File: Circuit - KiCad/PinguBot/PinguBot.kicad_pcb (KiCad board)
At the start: 2 copper layers, 96.3 x 104.8 mm, 26 parts, among them J1 Jack-DC, J2 Conn_01x08_Pin, J3 Conn_01x08_Pin, U1 LM386, U3 LM7805_TO220, U4 TSOP45xx, U5 ESP32_DEVKITC

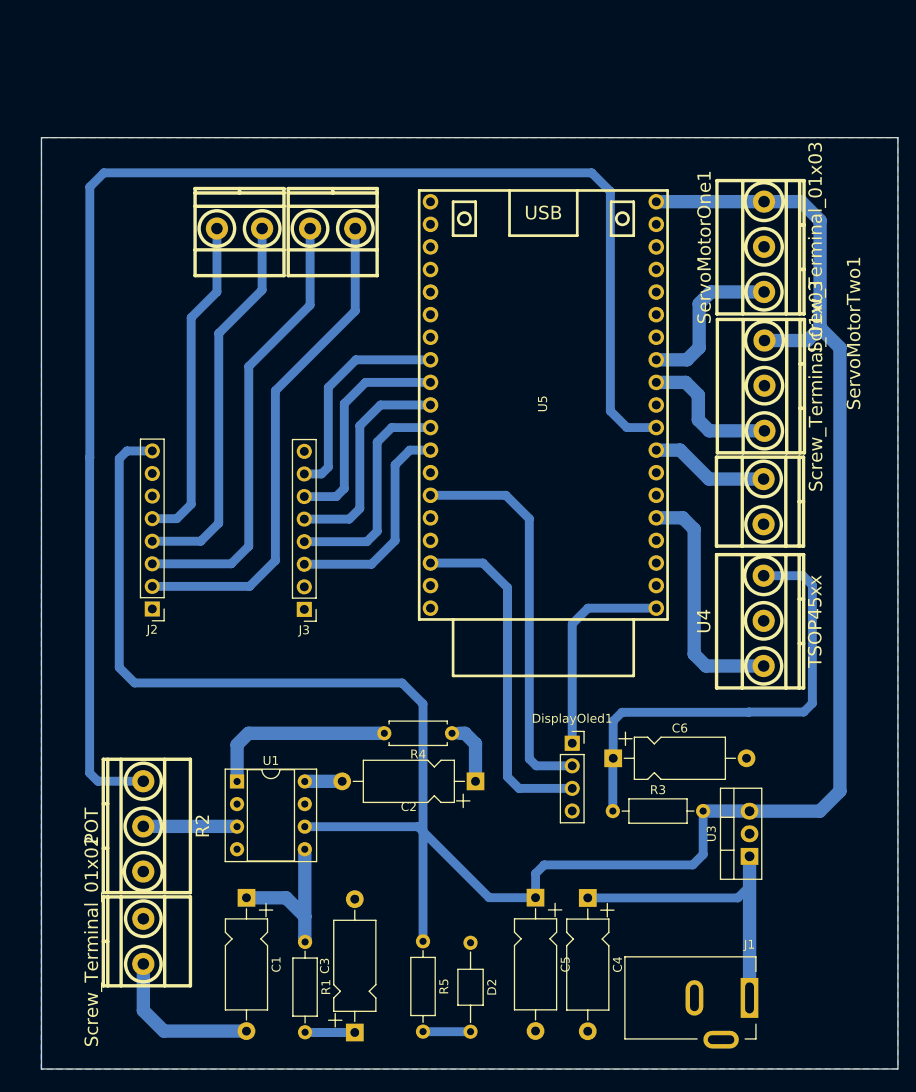
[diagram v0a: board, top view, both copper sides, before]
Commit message: Circuit Improvement
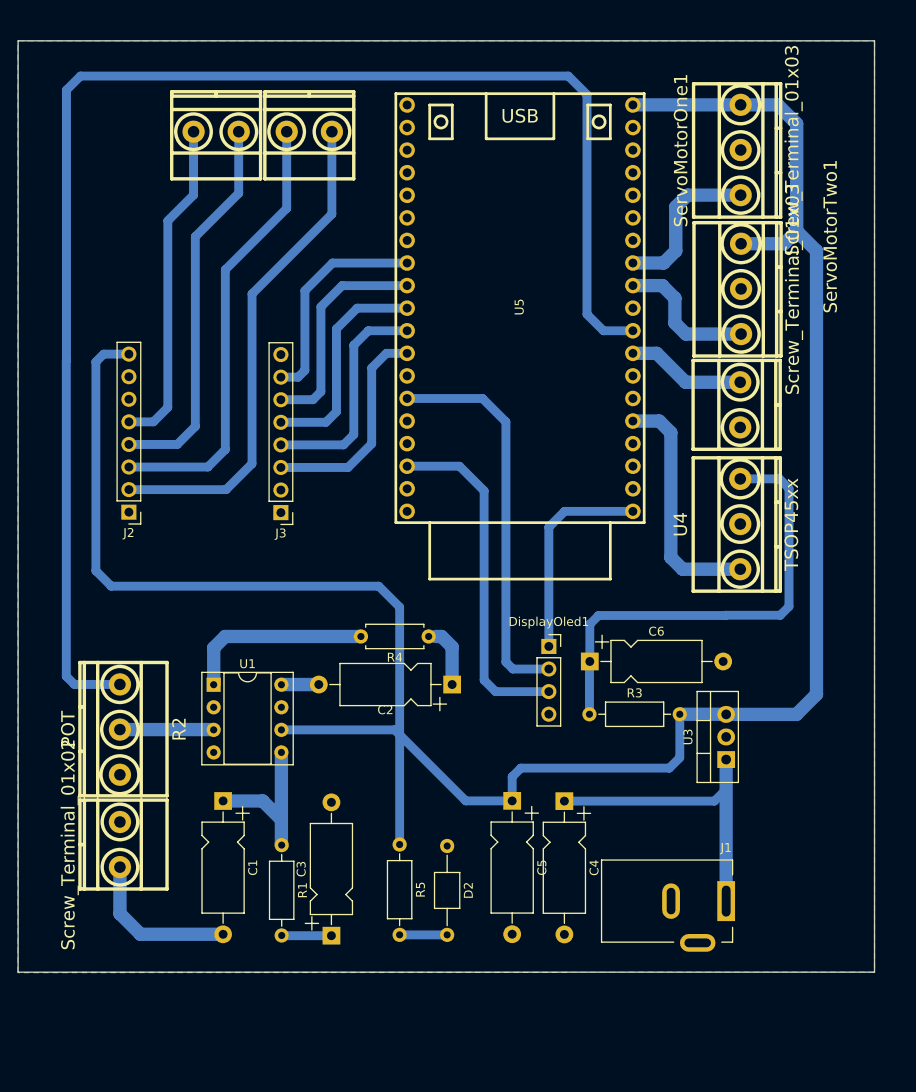
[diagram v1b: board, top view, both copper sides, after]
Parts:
- moved C3 11.2 mm to (71.4, 132.2)
- moved D2 11.2 mm to (84.4, 122.1)
- moved R1 11.2 mm to (65.8, 122.0)
- moved Speaker1 11.2 mm to (47.6, 121.9)
- moved C1 11.2 mm to (59.2, 117.0)
- moved J2 11.2 mm to (48.6, 84.5)
- moved U1 11.2 mm to (58.1, 103.9)
- moved C2 11.2 mm to (85.0, 103.9)
- moved C4 11.2 mm to (97.6, 117.0)
- moved C5 11.2 mm to (91.7, 117.0)
- moved C6 11.2 mm to (100.4, 101.3)
- moved DisplayOled1 11.2 mm to (95.8, 99.6)
- moved J3 11.2 mm to (65.7, 84.6)
- moved Microphone1 11.2 mm to (117.4, 72.4)
- moved R2 11.2 mm to (47.6, 109.0)
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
